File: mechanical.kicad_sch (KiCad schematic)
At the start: 0 parts

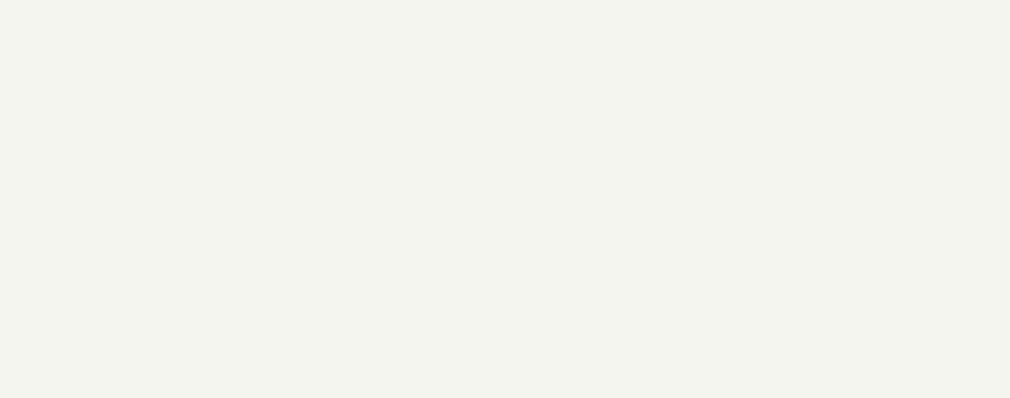
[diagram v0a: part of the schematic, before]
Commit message: SCH[Cleaning]:Updated Connectors not sure still, added sprate bat and ground connections, updated commincation conncetors. PCB[Layout]:Inital layout of compents need to fit on board size once tap connecton method is decided.
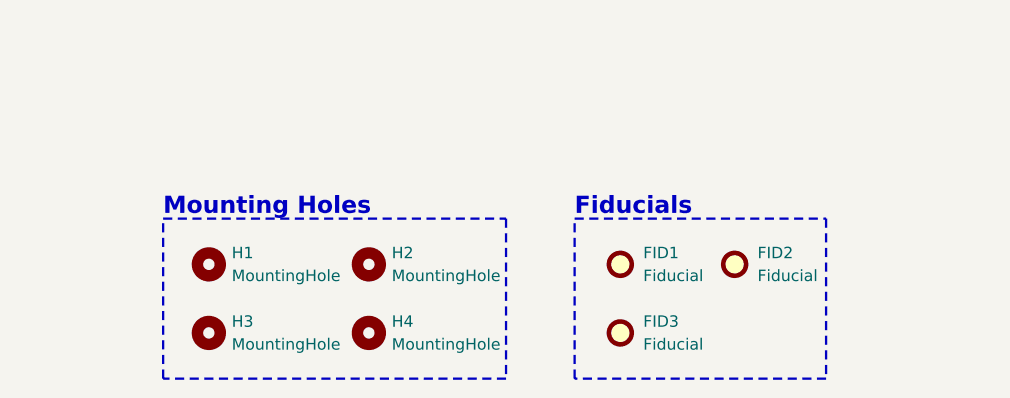
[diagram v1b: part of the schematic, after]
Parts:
- added FID1, FID2, FID3: Fiducial, Fiducial:Fiducial_0.5mm_Mask1mm, symbol Mechanical:Fiducial
- added H1, H2, H3, H4: MountingHole, MountingHole:MountingHole_3.2mm_M3, symbol Mechanical:MountingHole
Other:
- note added: "Fiducials"
- note added: "Mounting Holes"

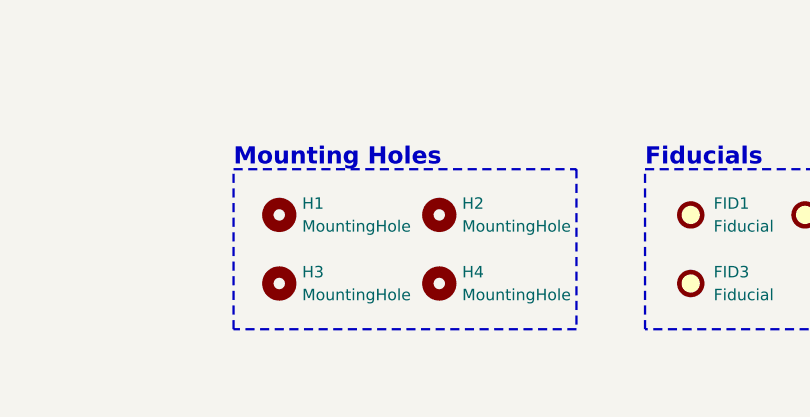
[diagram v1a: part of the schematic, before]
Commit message: PCB[DRC, Grouding]: Need to seprate top ground planes, and possibliy bring caps to top side, started adressing drc errors. To fix: Via sizing on bms chip, ground planes and senstive grounds, trace matching sens and bal, connector finilzation, temp routing, logos and other silk screen, test points, review!
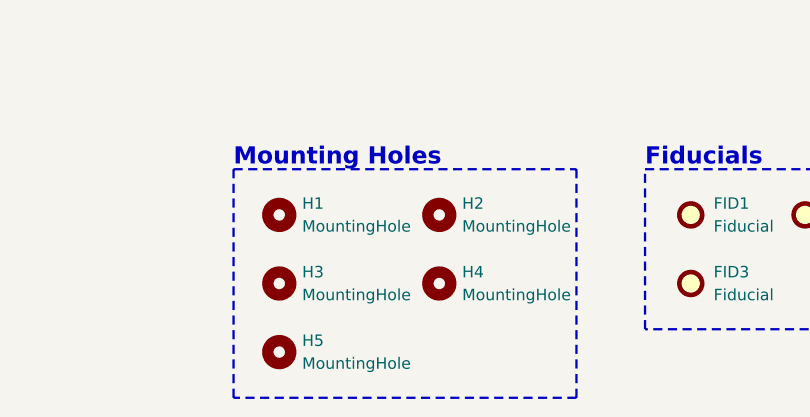
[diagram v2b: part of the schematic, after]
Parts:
- added H5: MountingHole, MountingHole:MountingHole_3.2mm_M3, symbol Mechanical:MountingHole
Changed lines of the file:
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@@
 	(rectangle
 		(start 101.6 83.82)
-		(end 139.7 101.6)
+		(end 139.7 109.22)
 		(stroke
 			(width 0.254)
@@
 					(unit 1)
 				)
+			)
+		)
+	)
+	(symbol
+		(lib_id "Mechanical:MountingHole")
+		(at 106.68 104.14 0)
+		(unit 1)
+		(body_style 1)
+		(exclude_from_sim no)
+		(in_bom no)
+		(on_board yes)
+		(in_pos_files yes)
+		(dnp no)
+		(fields_autoplaced yes)
+		(property "Reference" "H5"
+			(at 109.22 102.87 0)
+			(show_name no)
+			(do_not_autoplace no)
+			(effects
+				(font
+					(size 1.27 1.27)
+				)
+				(justify left)
+			)
+		)
+		(property "Value" "MountingHole"
+			(at 109.22 105.41 0)
+			(show_name no)
+			(do_not_autoplace no)
+			(effects
+				(font
+					(size 1.27 1.27)
+				)
+				(justify left)
+			)
+		)
+		(property "Footprint" "MountingHole:MountingHole_3.2mm_M3"
+			(at 106.68 104.14 0)
+			(hide yes)
+			(show_name no)
+			(do_not_autoplace no)
+			(effects
+				(font
+					(size 1.27 1.27)
+				)
+			)
+		)
+		(property "Datasheet" ""
+			(at 106.68 104.14 0)
+			(hide yes)
+			(show_name no)
+			(do_not_autoplace no)
+			(effects
+				(font
+					(size 1.27 1.27)
+				)
+			)
+		)
+		(property "Description" "Mounting Hole without connection"
+			(at 106.68 104.14 0)
+			(hide yes)
+			(show_name no)
+			(do_not_autoplace no)
+			(effects
+				(font
+					(size 1.27 1.27)
+				)
+			)
+		)
+		(instances
+			(project "bms_slave"
+				(path "/f9e05184-c88b-4a88-ae9c-ab2bdb32be7c/c5103ceb-5325-4a84-a025-9638a412984e/f4a7f626-808e-4d0f-b4d4-b24a2b39d327"
+					(reference "H5")
+					(unit 1)
+				)
